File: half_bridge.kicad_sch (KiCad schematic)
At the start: 31 parts, among them Q1 IGC019S06S1XTMA1, Q2 IGC019S06S1XTMA1, U19 NCS2220AMUT1G, U4 ACS37030LLZATR-065B3, U5 LMG1205YFXR

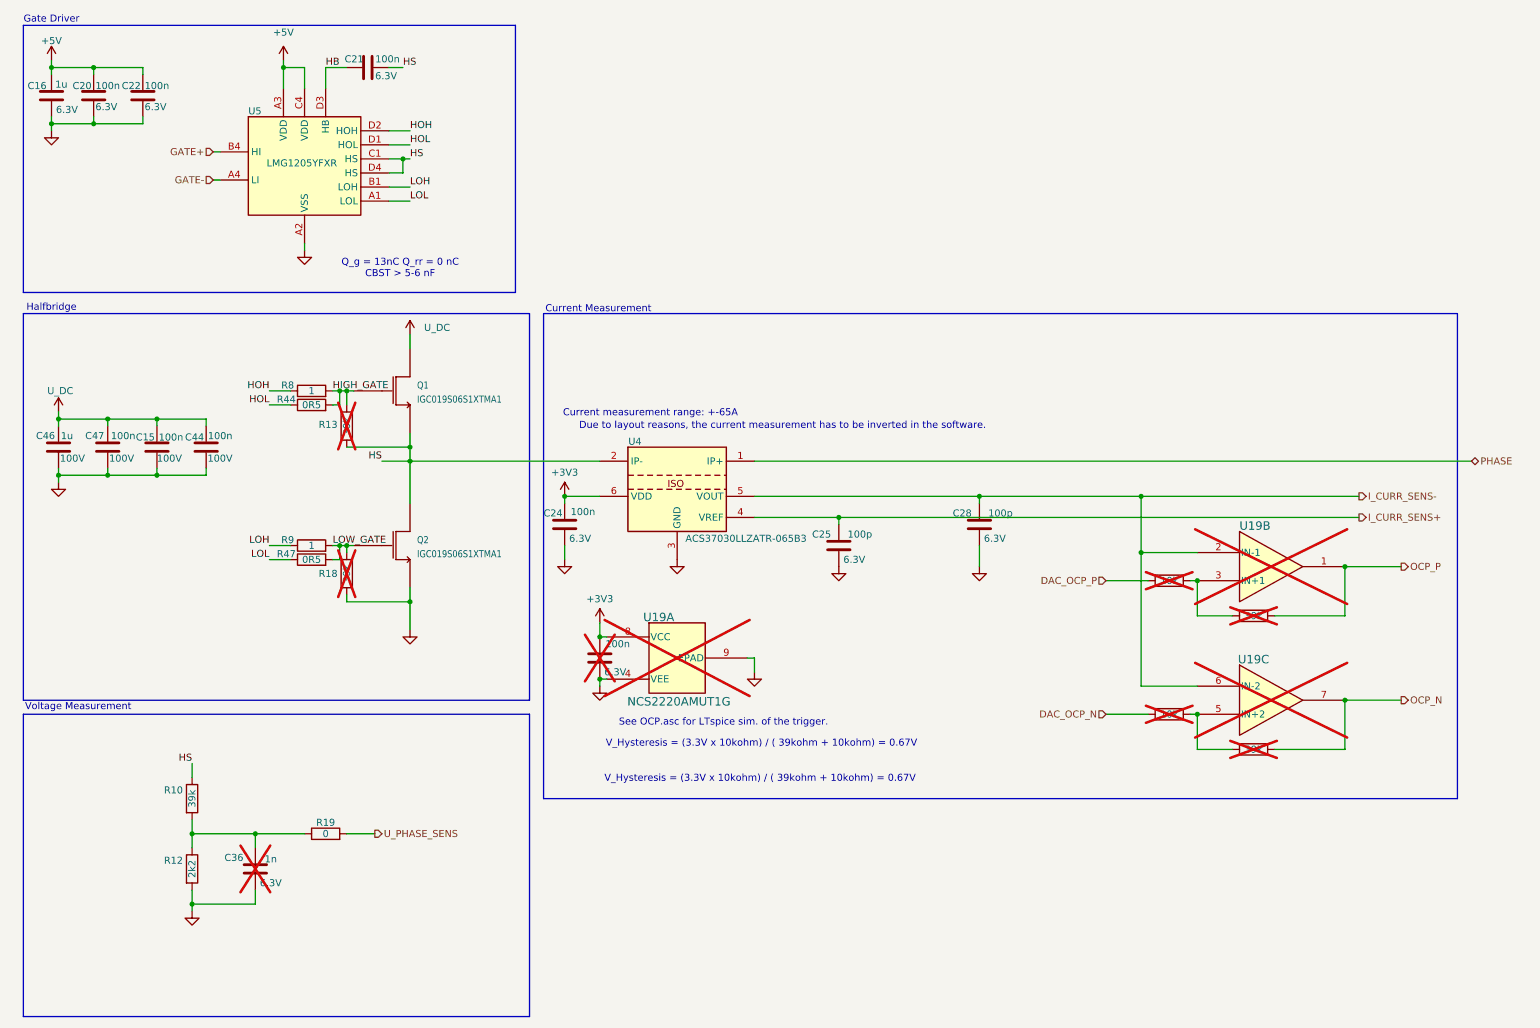
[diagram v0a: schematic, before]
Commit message: wip gate driver change
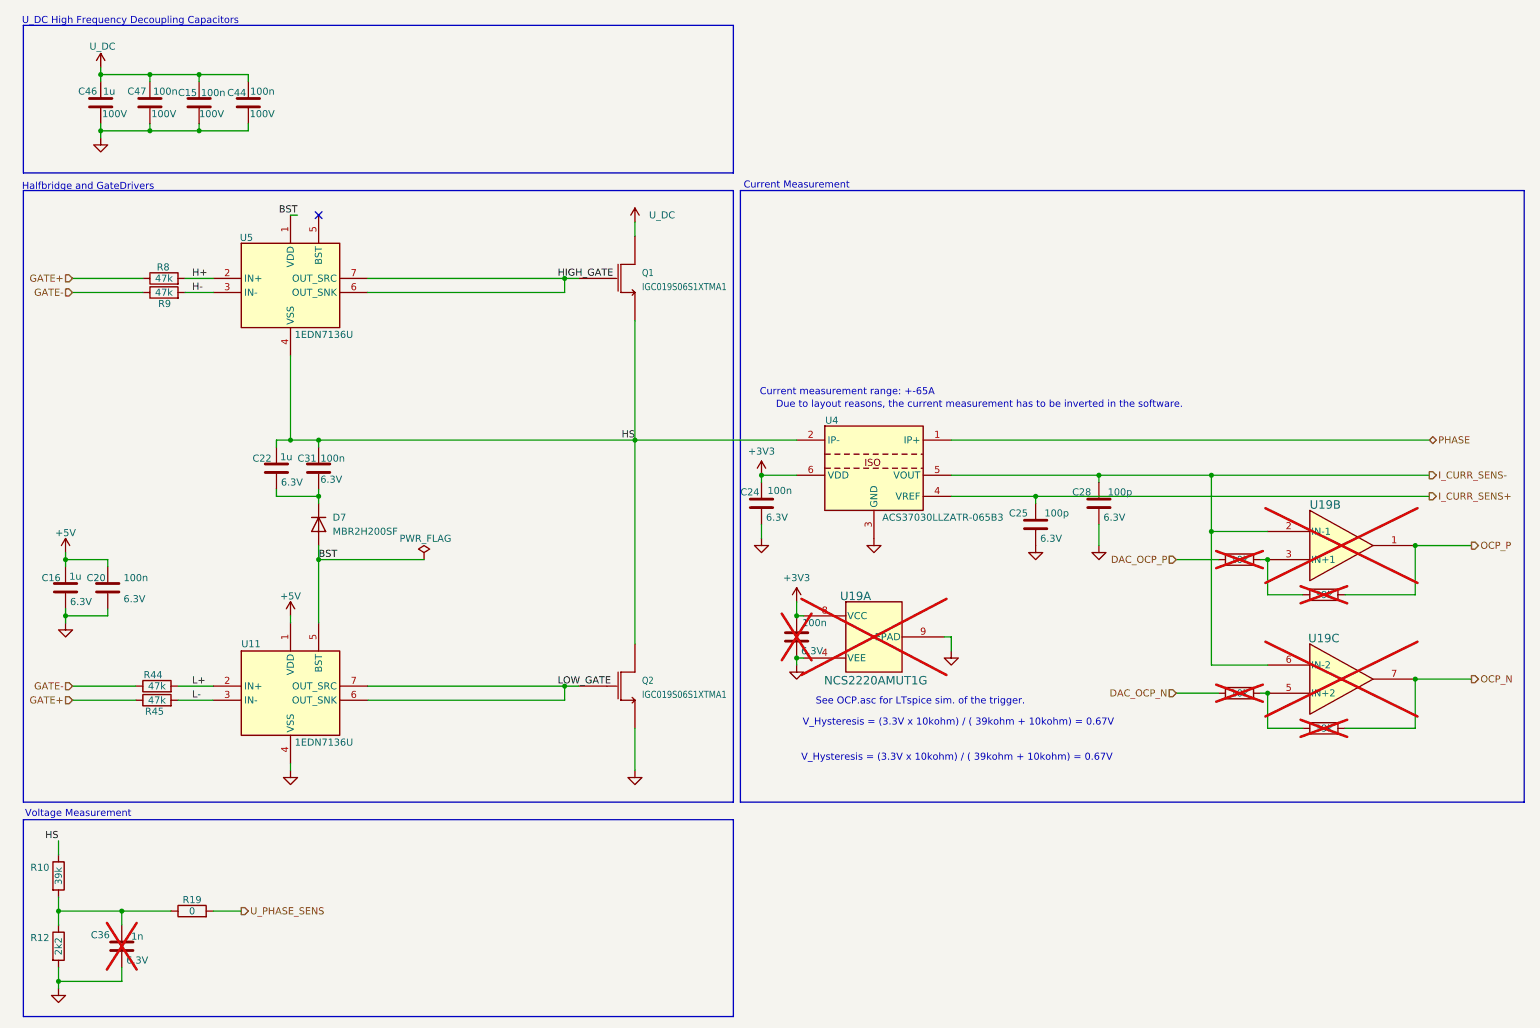
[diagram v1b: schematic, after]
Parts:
- removed C21: 0402B104K6R3CT, Capacitor_SMD:C_0402_1005Metric, symbol Device:C
- removed R13, R18: ~, Resistor_SMD:R_0402_1005Metric_Pad0.72x0.64mm_HandSolder, symbol Device:R
- removed R47: CSR0402FKR500, Resistor_SMD:R_0402_1005Metric, symbol Device:R
- removed U5: LMG1205YFXR, NanoGaN:BGA12C40P4X4_173X188X68, symbol NanoGaN:LMG1205YFXR
- added C31: 0402B104K6R3CT, Capacitor_SMD:C_0402_1005Metric, symbol Device:C
- added D7: MBR2H200SF, Diode_SMD:D_SOD-123F, symbol Device:D
- added R45: 0402WGF4702TCE, Resistor_SMD:R_0402_1005Metric, symbol Device:R
- added U11, U5: 1EDN7136U, NanoGaN:1EDN71X6U, symbol NanoGaN:1EDN7116U
- C22: value 0402B104K6R3CT -> CL05B105KQ5NQNC; Capacitance 100n -> 1u; LCSC C424821 -> C307427
- R44: value CSR0402FKR500 -> 0402WGF4702TCE; LCSC C346785 -> C25792; Resistance 0R5 -> 47k
- R8, R9: value CRCW04021R00FKEDHP -> 0402WGF4702TCE; LCSC C2077491 -> C25792; Resistance 1 -> 47k
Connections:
- net HOH is gone; now on net GATE+: R8.1
- net HOL is gone; now on net GATE-: R44.1
- net LOH is gone; now on net GATE-: R9.1
- net +5V: now also U11.1 (VDD); no longer C22.1
- net GATE+: now also R45.1
- net GND: now also U11.4 (VSS); no longer C22.2
- net HIGH_GATE: now also U5.6 (OUT_SNK), U5.7 (OUT_SRC); no longer R44.2, R8.2
- net HS: now also C22.1, C31.1, U5.4 (VSS)
- net LOW_GATE: now also U11.6 (OUT_SNK), U11.7 (OUT_SRC); no longer R9.2
- new net: C22.2, C31.2, D7.1 (K)
- new net BST: D7.2 (A), U11.5 (BST), U5.1 (VDD)
- new net H+: R8.2, U5.2 (IN+)
- new net H-: R9.2, U5.3 (IN-)
- new net L+: R44.2, U11.2 (IN+)
- new net L-: R45.2, U11.3 (IN-)
- no-connect marks 0 -> 1
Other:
- note added: "Halfbridge and GateDrivers"
- note added: "U_DC High Frequency Decoupling Capacitors"
- note removed: "Gate Driver"
- note removed: "Halfbridge"
- note removed: "Q_g = 13nC Q_rr = 0 nC CBST > 5-6 nF"
- moved on the sheet: C15, C16, C20, C24, C25, C28, C36, C44, C46, C47, Q1, Q2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
